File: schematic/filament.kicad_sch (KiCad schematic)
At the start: 14 parts, among them M1 Motor_DC, U1 MOC3021M, U2 MOC3021M

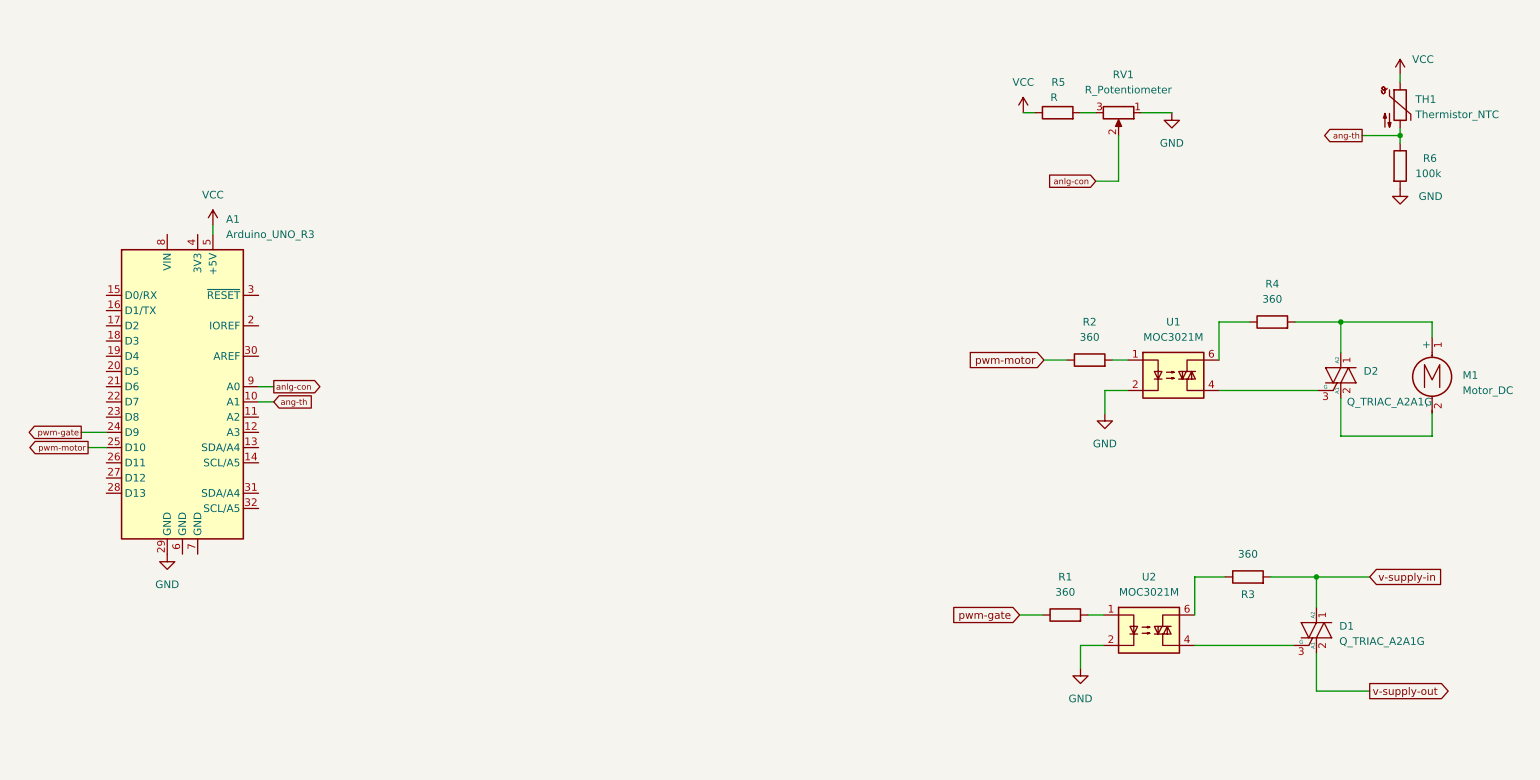
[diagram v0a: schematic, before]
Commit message: Updated schematic
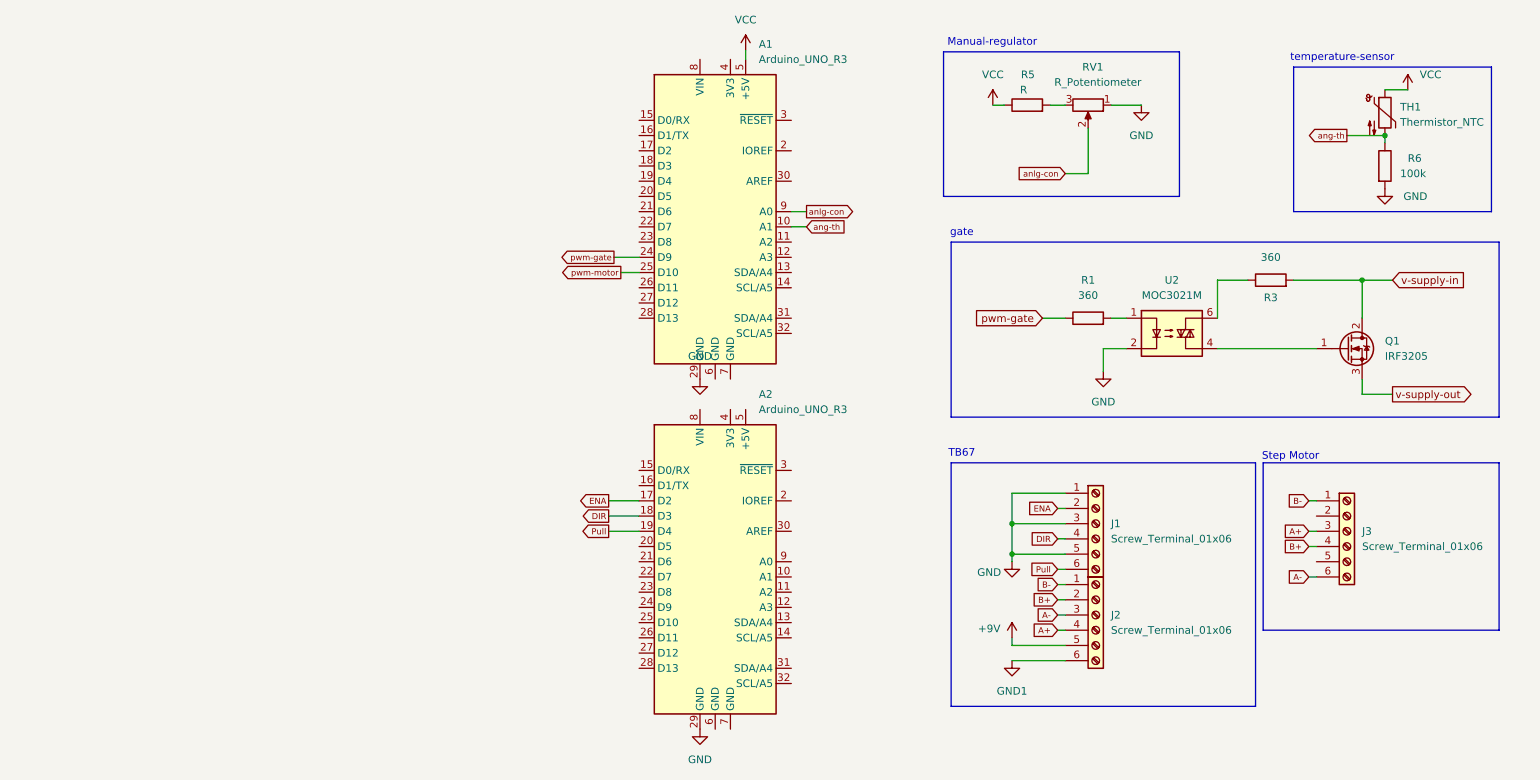
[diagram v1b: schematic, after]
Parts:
- removed D1, D2: Q_TRIAC_A2A1G, symbol Device:Q_TRIAC_A2A1G
- removed M1: Motor_DC, symbol Motor:Motor_DC
- removed R2, R4: 360, symbol Device:R
- removed U1: MOC3021M, symbol Relay_SolidState:MOC3021M
- added A2: Arduino_UNO_R3, Module:Arduino_UNO_R3, symbol MCU_Module:Arduino_UNO_R3
- added J1, J2, J3: Screw_Terminal_01x06, symbol Connector:Screw_Terminal_01x06
- added Q1: IRF3205, Package_TO_SOT_THT:TO-220-3_Vertical, symbol Transistor_FET:IRF3205
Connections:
- net GND: now also A2.29 (GND), J1.1 (Pin_1), J1.3 (Pin_3), J1.5 (Pin_5)
- net v-supply-in: now also Q1.2 (D)
- net v-supply-out: now also Q1.3 (S)
- net at U2.4: now also Q1.1 (G)
- new net +9V: J2.5 (Pin_5)
- new net A+: J2.4 (Pin_4), J3.3 (Pin_3)
- new net A-: J2.3 (Pin_3), J3.6 (Pin_6)
- new net B+: J2.2 (Pin_2), J3.4 (Pin_4)
- new net B-: J2.1 (Pin_1), J3.1 (Pin_1)
- new net DIR: A2.18 (D3), J1.4 (Pin_4)
- new net ENA: A2.17 (D2), J1.2 (Pin_2)
- new net GND1: J2.6 (Pin_6)
- new net Pull: A2.19 (D4), J1.6 (Pin_6)
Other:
- note added: "Manual-regulator"
- note added: "Step Motor"
- note added: "TB67"
- note added: "gate"
- note added: "temperature-sensor"
- moved on the sheet: A1, R1, R3, R5, R6, RV1, TH1, U2
